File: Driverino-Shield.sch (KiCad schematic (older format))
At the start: 55 parts, among them P1 Power, P10 MOT, P11 HALL, P2 Analog, P3 Digital, P4 Digital, P5 CONN_01X01, P6 CONN_01X01, P7 CONN_01X01, P8 CONN_01X01, P9 PWR, U1 MCT8316Z

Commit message: Update
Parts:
- added JP2: VCC_SEL, Connector_PinHeader_1.27mm:PinHeader_1x02_P1.27mm_Vertical, symbol Device:Jumper
- C1, C10, C11, C12, C3, C4, C5, C6, C7, C8, C9: symbol device:C -> Driverino-Shield-rescue:C-device
- C2: symbol device:CP1 -> Driverino-Shield-rescue:CP1-device
- D1, D2, D3, D4: symbol device:LED -> Driverino-Shield-rescue:LED-device
- D5: symbol device:ZENER -> Driverino-Shield-rescue:ZENER-device
- F1: symbol device:FUSE -> Driverino-Shield-rescue:FUSE-device
- JP1: footprint Driverino-Shield:3JUMPER_0603 -> Connector_PinHeader_1.27mm:PinHeader_1x03_P1.27mm_Vertical; symbol device:JUMPER3 -> Driverino-Shield-rescue:JUMPER3-device
- L1: renamed from L2; symbol device:INDUCTOR_SMALL -> Driverino-Shield-rescue:INDUCTOR_SMALL-device
- P10: symbol conn:CONN_3 -> Driverino-Shield-rescue:CONN_3-conn
- P11: symbol conn:CONN_8 -> Driverino-Shield-rescue:CONN_8-conn
- P9: symbol conn:CONN_2 -> Driverino-Shield-rescue:CONN_2-conn
- R1, R10, R11, R12, R13, R14, R15, R16, R17, R18, R19, R2, R20, R21, R22, R23, R3, R4, R5, R6, R7, R8, R9: symbol device:R -> Driverino-Shield-rescue:R-device
- U1: symbol texas2:MCT8316Z -> Driverino-Shield-rescue:MCT8316Z-texas2
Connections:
- wire segments 237 -> 239

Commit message: Routing completed
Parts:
- C10, C11, C12, C4, C6: footprint Driverino-Shield:C_0603_1608Metric -> Capacitor_SMD:C_0402_1005Metric
- C3: footprint Driverino-Shield:C_0603_1608Metric -> Capacitor_SMD:C_1206_3216Metric
- JP2: symbol Device:Jumper -> Driverino-Shield-rescue:Jumper-Device
- R18, R19, R20, R21, R22, R23: footprint Resistor_SMD:R_0603_1608Metric -> Resistor_SMD:R_0402_1005Metric
- U1: symbol Driverino-Shield-rescue:MCT8316Z-texas2 -> Driverino-Shield-rescue:MCT8316Z-texas2-Driverino-Shield-rescue
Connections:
- net V: now also U1.16 (OUTB); no longer U1.16, (OUTB)

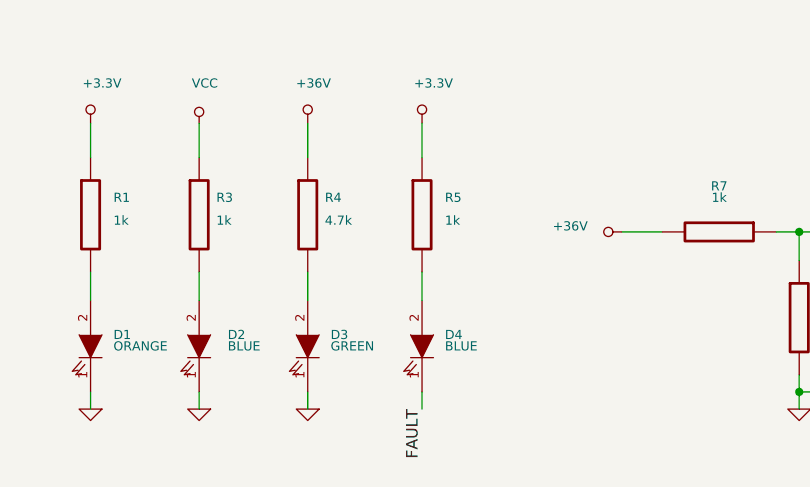
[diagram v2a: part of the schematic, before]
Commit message: Update
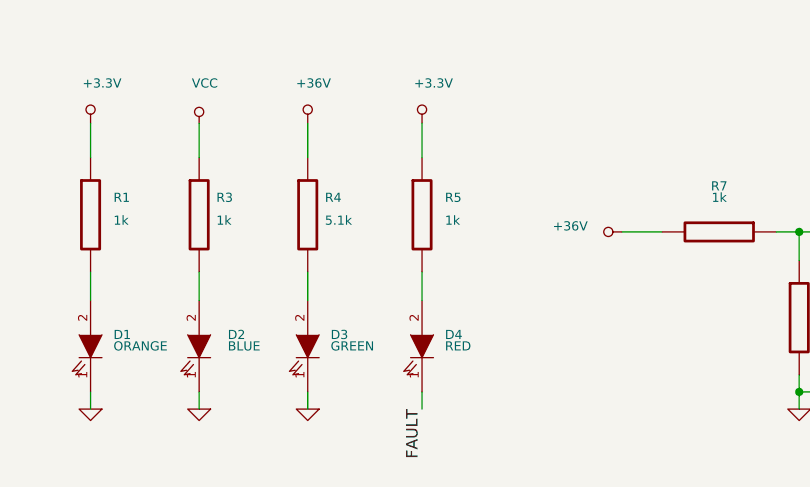
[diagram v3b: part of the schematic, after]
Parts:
- C1: Manufacturer (none) -> KEMET; Provider (none) -> RS; ProviderCode (none) -> 802-9967; manf# (none) -> C1206C226M8RACTU; mpn (none) -> C1206C226M8RACTU
- C10, C11, C12, C4: Manufacturer (none) -> TDK; Provider (none) -> RS; ProviderCode (none) -> 915-5635; manf# (none) -> CGA2B3X7R1V104K050BB; mpn (none) -> CGA2B3X7R1V104K050BB
- C2: Manufacturer (none) -> Panasonic; Provider (none) -> Mouser; ProviderCode (none) -> 667-EEE-FTV151XAV; manf# (none) -> EEE-FTV151XAV; mpn (none) -> EEE-FTV151XAV
- C3: Manufacturer (none) -> TDK; Provider (none) -> RS; ProviderCode (none) -> 915-5354; manf# (none) -> CGA5L1X7R1V106K160AE; mpn (none) -> CGA5L1X7R1V106K160AE
- C5, C7: Manufacturer (none) -> Yageo; Provider (none) -> RS; ProviderCode (none) -> 200-6596; manf# (none) -> CC0603KRX7R9BB105; mpn (none) -> CC0603KRX7R9BB105
- C6: Manufacturer (none) -> Murata; Provider (none) -> RS; ProviderCode (none) -> 723-4954; manf# (none) -> GCM155R71H103KA55D; mpn (none) -> GCM155R71H103KA55D
- C8, C9: Manufacturer (none) -> TDK; Provider (none) -> RS; ProviderCode (none) -> 788-2985; manf# (none) -> CGA3E2X7R1H104K080AA; mpn (none) -> CGA3E2X7R1H104K080AA
- D4: value BLUE -> RED
- D5: Manufacturer (none) -> Taiwan Semiconductor; Provider (none) -> Mouser; ProviderCode (none) -> 821-TSZU52C5V1RGG; manf# (none) -> TSZU52C5V1 RGG; mpn (none) -> TSZU52C5V1 RGG
- F1: Manufacturer (none) -> Bourns; Provider (none) -> Mouser; ProviderCode (none) -> 652-MF-ASML020/6-2; manf# (none) -> MF-ASML020/6-2; mpn (none) -> MF-ASML020/6-2
- JP1: Manufacturer (none) -> Samtec; Provider (none) -> Mouser; manf# (none) -> TMS-103-01-G-S; mpn (none) -> TMS-103-01-G-S
- JP2: Manufacturer (none) -> Samtec; Provider (none) -> Mouser; manf# (none) -> TMS-102-01-G-S; mpn (none) -> TMS-102-01-G-S
- L1: Manufacturer (none) -> Taiyo Yuden; Provider (none) -> Mouser; ProviderCode (none) -> 963-CBC3225T470KRV; manf# (none) -> CBC3225T470KRV; mpn (none) -> CBC3225T470KRV
- P1, P4: Manufacturer (none) -> Samtec; manf# (none) -> SSW-108-03-G-S; mpn (none) -> SSW-108-03-G-S
- P10: Manufacturer (none) -> Molex; manf# (none) -> 39773-0003; mpn (none) -> 39773-0003
- P11: Manufacturer (none) -> Molex; manf# (none) -> 53047-0810; mpn (none) -> 53047-0810
- P2: Manufacturer (none) -> Samtec; manf# (none) -> SSW-106-03-G-S; mpn (none) -> SSW-106-03-G-S
- P3: Manufacturer (none) -> Samtec; manf# (none) -> SSW-110-03-G-S; mpn (none) -> SSW-110-03-G-S
- P9: Manufacturer (none) -> Molex; manf# (none) -> 39773-0002; mpn (none) -> 39773-0002
- R1, R13, R3, R5, R7, R8: Manufacturer (none) -> Vishay; Provider (none) -> Mouser; ProviderCode (none) -> 71-CRCW06031K00FKEAC; manf# (none) -> CRCW06031K00FKEAC; mpn (none) -> CRCW06031K00FKEAC
- R10, R11, R12, R14, R15, R16, R17, R9: Manufacturer (none) -> Vishay; Provider (none) -> Mouser; ProviderCode (none) -> 71-CRCW06030000Z0EBC; manf# (none) -> CRCW06030000Z0EBC; mpn (none) -> CRCW06030000Z0EBC
- R18, R20, R22: Manufacturer (none) -> Vishay; Provider (none) -> Mouser; ProviderCode (none) -> 71-CRCW040210K0JNEDC; manf# (none) -> CRCW040210K0JNEDC; mpn (none) -> CRCW040210K0JNEDC
- R19, R21, R23: Manufacturer (none) -> Vishay; Provider (none) -> Mouser; ProviderCode (none) -> 71-RCC04020000Z0ED; manf# (none) -> RCC04020000Z0ED; mpn (none) -> RCC04020000Z0ED
- R2, R6: Manufacturer (none) -> Rohm; Provider (none) -> Mouser; ProviderCode (none) -> 755-ESR03EZPF5101; manf# (none) -> ESR03EZPF5101; mpn (none) -> ESR03EZPF5101
- R4: value 4.7k -> 5.1k; Manufacturer (none) -> Rohm; Provider (none) -> Mouser; ProviderCode (none) -> 755-ESR03EZPF5101; manf# (none) -> ESR03EZPF5101; mpn (none) -> ESR03EZPF5101
- U1: Manufacturer (none) -> TI; manf# (none) -> MCT8316Z; mpn (none) -> MCT8316Z

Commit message: .tsv file generated
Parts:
- D1: Manufacturer (none) -> 654-5795; Provider (none) -> RS; ProviderCode (none) -> OSRAM Opto; manf# (none) -> LO Q976; mpn (none) -> LO Q976
- D2: Manufacturer (none) -> 697-3610; Provider (none) -> RS; ProviderCode (none) -> OSRAM Opto; manf# (none) -> LB Q39G-N1OO-35-1; mpn (none) -> LB Q39G-N1OO-35-1
- D3: Manufacturer (none) -> 697-3715; Provider (none) -> RS; ProviderCode (none) -> OSRAM Opto; manf# (none) -> LT Q39G-Q1OO-25-1; mpn (none) -> LT Q39G-Q1OO-25-1
- D4: Manufacturer (none) -> 466-3728; Provider (none) -> RS; ProviderCode (none) -> Kingbright; manf# (none) -> KP-1608SRC-PRV; mpn (none) -> KP-1608SRC-PRV
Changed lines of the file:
@@
 F 2 "Driverino-Shield:LED_0603_1608Metric" H 5200 9200 60  0001 C CNN
 F 3 "" H 5200 9200 60  0000 C CNN
+F 4 "654-5795" H 5200 9200 50  0001 C CNN "Manufacturer"
+F 5 "RS" H 5200 9200 50  0001 C CNN "Provider"
+F 6 "OSRAM Opto" H 5200 9200 50  0001 C CNN "ProviderCode"
+F 7 "LO Q976" H 5200 9200 50  0001 C CNN "manf#"
+F 8 "LO Q976" H 5200 9200 50  0001 C CNN "mpn"
 	1    5200 9200
 	0    1    1    0
@@
 F 2 "Driverino-Shield:LED_0603_1608Metric" H 5675 9200 60  0001 C CNN
 F 3 "" H 5675 9200 60  0000 C CNN
+F 4 "697-3610" H 5675 9200 50  0001 C CNN "Manufacturer"
+F 5 "RS" H 5675 9200 50  0001 C CNN "Provider"
+F 6 "OSRAM Opto" H 5675 9200 50  0001 C CNN "ProviderCode"
+F 7 "LB Q39G-N1OO-35-1" H 5675 9200 50  0001 C CNN "manf#"
+F 8 "LB Q39G-N1OO-35-1" H 5675 9200 50  0001 C CNN "mpn"
 	1    5675 9200
 	0    1    1    0
@@
 F 2 "Driverino-Shield:LED_0603_1608Metric" H 6150 9200 60  0001 C CNN
 F 3 "" H 6150 9200 60  0000 C CNN
+F 4 "697-3715" H 6150 9200 50  0001 C CNN "Manufacturer"
+F 5 "RS" H 6150 9200 50  0001 C CNN "Provider"
+F 6 "OSRAM Opto" H 6150 9200 50  0001 C CNN "ProviderCode"
+F 7 "LT Q39G-Q1OO-25-1" H 6150 9200 50  0001 C CNN "manf#"
+F 8 "LT Q39G-Q1OO-25-1" H 6150 9200 50  0001 C CNN "mpn"
 	1    6150 9200
 	0    1    1    0
@@
 F 2 "Driverino-Shield:LED_0603_1608Metric" H 6650 9200 60  0001 C CNN
 F 3 "" H 6650 9200 60  0000 C CNN
+F 4 "466-3728" H 6650 9200 50  0001 C CNN "Manufacturer"
+F 5 "RS" H 6650 9200 50  0001 C CNN "Provider"
+F 6 "Kingbright" H 6650 9200 50  0001 C CNN "ProviderCode"
+F 7 "KP-1608SRC-PRV" H 6650 9200 50  0001 C CNN "manf#"
+F 8 "KP-1608SRC-PRV" H 6650 9200 50  0001 C CNN "mpn"
 	1    6650 9200
 	0    1    1    0

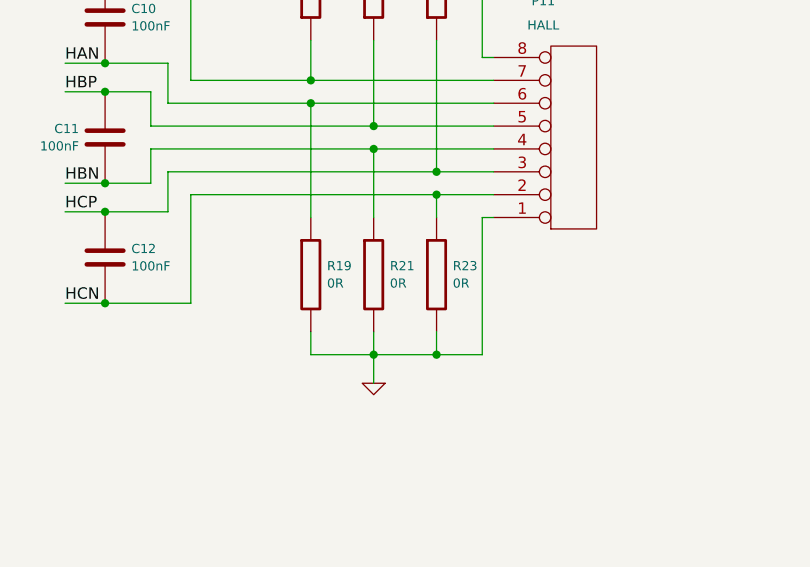
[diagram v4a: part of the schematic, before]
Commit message: Update BOM
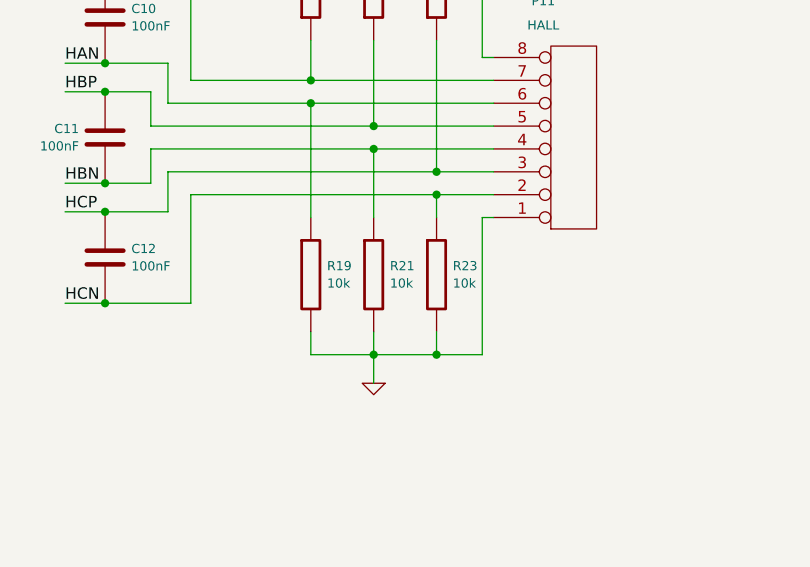
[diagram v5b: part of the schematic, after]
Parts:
- C10, C11, C12, P5, P6, P7, P8, R18, R20, R22: DNP (none) -> 1
- R19, R21, R23: value 0R -> 10k; DNP (none) -> 1; ProviderCode 71-RCC04020000Z0ED -> 71-CRCW040210K0JNEDC; manf# RCC04020000Z0ED -> CRCW040210K0JNEDC; mpn RCC04020000Z0ED -> CRCW040210K0JNEDC
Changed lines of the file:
@@
 F 2 "Socket_Arduino_Uno:Arduino_1pin" H 15571 724 20  0000 C CNN
 F 3 "" H 15650 650 50  0000 C CNN
+F 4 "1" H 15650 650 50  0001 C CNN "DNP"
 	1    15650 650
 	0    -1   -1   0
@@
 F 2 "Socket_Arduino_Uno:Arduino_1pin" H 15750 650 20  0001 C CNN
 F 3 "" H 15750 650 50  0000 C CNN
+F 4 "1" H 15750 650 50  0001 C CNN "DNP"
 	1    15750 650
 	0    -1   -1   0
@@
 F 2 "Socket_Arduino_Uno:Arduino_1pin" V 15850 650 20  0001 C CNN
 F 3 "" H 15850 650 50  0000 C CNN
+F 4 "1" H 15850 650 50  0001 C CNN "DNP"
 	1    15850 650
 	0    -1   -1   0
@@
 F 2 "Socket_Arduino_Uno:Arduino_1pin" H 15874 572 20  0000 C CNN
 F 3 "" H 15950 650 50  0000 C CNN
+F 4 "1" H 15950 650 50  0001 C CNN "DNP"
 	1    15950 650
 	0    -1   -1   0
@@
 F 7 "CGA2B3X7R1V104K050BB" H 13050 6425 50  0001 C CNN "manf#"
 F 8 "CGA2B3X7R1V104K050BB" H 13050 6425 50  0001 C CNN "mpn"
+F 9 "1" H 13050 6425 50  0001 C CNN "DNP"
 	1    13050 6425
 	-1   0    0    1
@@
 F 7 "CGA2B3X7R1V104K050BB" H 13050 6950 50  0001 C CNN "manf#"
 F 8 "CGA2B3X7R1V104K050BB" H 13050 6950 50  0001 C CNN "mpn"
+F 9 "1" H 13050 6950 50  0001 C CNN "DNP"
 	1    13050 6950
 	-1   0    0    1
@@
 F 7 "CGA2B3X7R1V104K050BB" H 13050 7475 50  0001 C CNN "manf#"
 F 8 "CGA2B3X7R1V104K050BB" H 13050 7475 50  0001 C CNN "mpn"
+F 9 "1" H 13050 7475 50  0001 C CNN "DNP"
 	1    13050 7475
 	-1   0    0    1
@@
 P 14225 7550
 F 0 "R21" H 14296 7588 40  0000 L CNN
-F 1 "0R" H 14296 7512 40  0000 L CNN
+F 1 "10k" H 14296 7512 40  0000 L CNN
 F 2 "Resistor_SMD:R_0402_1005Metric" V 14155 7550 30  0001 C CNN
 F 3 "" H 14225 7550 30  0000 C CNN
 F 4 "Vishay" H 14225 7550 50  0001 C CNN "Manufacturer"
 F 5 "Mouser" H 14225 7550 50  0001 C CNN "Provider"
-F 6 "71-RCC04020000Z0ED" H 14225 7550 50  0001 C CNN "ProviderCode"
-F 7 "RCC04020000Z0ED" H 14225 7550 50  0001 C CNN "manf#"
-F 8 "RCC04020000Z0ED" H 14225 7550 50  0001 C CNN "mpn"
+F 6 "71-CRCW040210K0JNEDC" H 14225 7550 50  0001 C CNN "ProviderCode"
+F 7 "CRCW040210K0JNEDC" H 14225 7550 50  0001 C CNN "manf#"
+F 8 "CRCW040210K0JNEDC" H 14225 7550 50  0001 C CNN "mpn"
+F 9 "1" H 14225 7550 50  0001 C CNN "DNP"
 	1    14225 7550
 	1    0    0    -1
@@
 P 13950 7550
 F 0 "R19" H 14021 7588 40  0000 L CNN
-F 1 "0R" H 14021 7512 40  0000 L CNN
+F 1 "10k" H 14021 7512 40  0000 L CNN
 F 2 "Resistor_SMD:R_0402_1005Metric" V 13880 7550 30  0001 C CNN
 F 3 "" H 13950 7550 30  0000 C CNN
 F 4 "Vishay" H 13950 7550 50  0001 C CNN "Manufacturer"
 F 5 "Mouser" H 13950 7550 50  0001 C CNN "Provider"
-F 6 "71-RCC04020000Z0ED" H 13950 7550 50  0001 C CNN "ProviderCode"
-F 7 "RCC04020000Z0ED" H 13950 7550 50  0001 C CNN "manf#"
-F 8 "RCC04020000Z0ED" H 13950 7550 50  0001 C CNN "mpn"
+F 6 "71-CRCW040210K0JNEDC" H 13950 7550 50  0001 C CNN "ProviderCode"
+F 7 "CRCW040210K0JNEDC" H 13950 7550 50  0001 C CNN "manf#"
+F 8 "CRCW040210K0JNEDC" H 13950 7550 50  0001 C CNN "mpn"
+F 9 "1" H 13950 7550 50  0001 C CNN "DNP"
 	1    13950 7550
 	1    0    0    -1
@@
 P 14500 7550
 F 0 "R23" H 14571 7588 40  0000 L CNN
-F 1 "0R" H 14571 7512 40  0000 L CNN
+F 1 "10k" H 14571 7512 40  0000 L CNN
 F 2 "Resistor_SMD:R_0402_1005Metric" V 14430 7550 30  0001 C CNN
 F 3 "" H 14500 7550 30  0000 C CNN
 F 4 "Vishay" H 14500 7550 50  0001 C CNN "Manufacturer"
 F 5 "Mouser" H 14500 7550 50  0001 C CNN "Provider"
-F 6 "71-RCC04020000Z0ED" H 14500 7550 50  0001 C CNN "ProviderCode"
-F 7 "RCC04020000Z0ED" H 14500 7550 50  0001 C CNN "manf#"
-F 8 "RCC04020000Z0ED" H 14500 7550 50  0001 C CNN "mpn"
+F 6 "71-CRCW040210K0JNEDC" H 14500 7550 50  0001 C CNN "ProviderCode"
+F 7 "CRCW040210K0JNEDC" H 14500 7550 50  0001 C CNN "manf#"
+F 8 "CRCW040210K0JNEDC" H 14500 7550 50  0001 C CNN "mpn"
+F 9 "1" H 14500 7550 50  0001 C CNN "DNP"
 	1    14500 7550
 	1    0    0    -1
@@
 F 7 "CRCW040210K0JNEDC" H 14500 6275 50  0001 C CNN "manf#"
 F 8 "CRCW040210K0JNEDC" H 14500 6275 50  0001 C CNN "mpn"
+F 9 "1" H 14500 6275 50  0001 C CNN "DNP"
 	1    14500 6275
 	1    0    0    1
@@
 F 7 "CRCW040210K0JNEDC" H 14225 6275 50  0001 C CNN "manf#"
 F 8 "CRCW040210K0JNEDC" H 14225 6275 50  0001 C CNN "mpn"
+F 9 "1" H 14225 6275 50  0001 C CNN "DNP"
 	1    14225 6275
 	1    0    0    1
@@
 F 7 "CRCW040210K0JNEDC" H 13950 6275 50  0001 C CNN "manf#"
 F 8 "CRCW040210K0JNEDC" H 13950 6275 50  0001 C CNN "mpn"
+F 9 "1" H 13950 6275 50  0001 C CNN "DNP"
 	1    13950 6275
 	1    0    0    1

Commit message: BOM Update
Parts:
- C1: Manf (none) -> KEMET; Manufacturer KEMET -> (none); OrderCode (none) -> 802-9967; ProviderCode 802-9967 -> (none)
- C10, C11, C12, C4: Manf (none) -> TDK; Manufacturer TDK -> (none); OrderCode (none) -> 915-5635; ProviderCode 915-5635 -> (none)
- C2: Manf (none) -> Panasonic; Manufacturer Panasonic -> (none); OrderCode (none) -> 667-EEE-FTV151XAV; ProviderCode 667-EEE-FTV151XAV -> (none)
- C3: Manf (none) -> TDK; Manufacturer TDK -> (none); OrderCode (none) -> 915-5354; ProviderCode 915-5354 -> (none)
- C5, C7: Manf (none) -> Yageo; Manufacturer Yageo -> (none); OrderCode (none) -> 200-6596; ProviderCode 200-6596 -> (none)
- C6: Manf (none) -> Murata; Manufacturer Murata -> (none); OrderCode (none) -> 723-4954; ProviderCode 723-4954 -> (none)
- C8, C9: Manf (none) -> TDK; Manufacturer TDK -> (none); OrderCode (none) -> 788-2985; ProviderCode 788-2985 -> (none)
- D1: Manf (none) -> OSRAM Opto; Manufacturer 654-5795 -> (none); OrderCode (none) -> 654-5795; ProviderCode OSRAM Opto -> (none)
- D2: Manf (none) -> OSRAM Opto; Manufacturer 697-3610 -> (none); OrderCode (none) -> 697-3610; ProviderCode OSRAM Opto -> (none)
- D3: Manf (none) -> OSRAM Opto; Manufacturer 697-3715 -> (none); OrderCode (none) -> 697-3715; ProviderCode OSRAM Opto -> (none)
- D4: Manf (none) -> Kingbright; Manufacturer 466-3728 -> (none); OrderCode (none) -> 466-3728; ProviderCode Kingbright -> (none)
- D5: Manf (none) -> Taiwan Semiconductor; Manufacturer Taiwan Semiconductor -> (none); OrderCode (none) -> 821-TSZU52C5V1RGG; ProviderCode 821-TSZU52C5V1RGG -> (none)
- F1: Manf (none) -> Bourns; Manufacturer Bourns -> (none); OrderCode (none) -> 652-MF-ASML020/6-2; ProviderCode 652-MF-ASML020/6-2 -> (none)
- JP1, JP2, P1, P2, P3, P4: Manf (none) -> Samtec; Manufacturer Samtec -> (none)
- L1: Manf (none) -> Taiyo Yuden; Manufacturer Taiyo Yuden -> (none); OrderCode (none) -> 963-CBC3225T470KRV; ProviderCode 963-CBC3225T470KRV -> (none)
- P10, P11, P9: Manf (none) -> Molex; Manufacturer Molex -> (none)
- R1, R13, R3, R5, R7, R8: Manf (none) -> Vishay; Manufacturer Vishay -> (none); OrderCode (none) -> 71-CRCW06031K00FKEAC; ProviderCode 71-CRCW06031K00FKEAC -> (none)
- R10, R11, R12, R14, R15, R16, R17, R9: Manf (none) -> Vishay; Manufacturer Vishay -> (none); OrderCode (none) -> 71-CRCW06030000Z0EBC; ProviderCode 71-CRCW06030000Z0EBC -> (none)
- R18, R19, R20, R21, R22, R23: Manf (none) -> Vishay; Manufacturer Vishay -> (none); OrderCode (none) -> 71-CRCW040210K0JNEDC; ProviderCode 71-CRCW040210K0JNEDC -> (none)
- R2, R4, R6: Manf (none) -> Rohm; Manufacturer Rohm -> (none); OrderCode (none) -> 755-ESR03EZPF5101; ProviderCode 755-ESR03EZPF5101 -> (none)
- U1: Manf (none) -> TI; Manufacturer TI -> (none)

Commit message: Updated BOM
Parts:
- C10, C11, C12, P5, P6, P7, P8, R18, R19, R20, R21, R22, R23: DNF (none) -> 1; DNP 1 -> (none)
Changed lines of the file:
@@
 F 2 "Socket_Arduino_Uno:Arduino_1pin" H 15571 724 20  0000 C CNN
 F 3 "" H 15650 650 50  0000 C CNN
-F 4 "1" H 15650 650 50  0001 C CNN "DNP"
+F 4 "1" H 15650 650 50  0001 C CNN "DNF"
 	1    15650 650
 	0    -1   -1   0
@@
 F 2 "Socket_Arduino_Uno:Arduino_1pin" H 15750 650 20  0001 C CNN
 F 3 "" H 15750 650 50  0000 C CNN
-F 4 "1" H 15750 650 50  0001 C CNN "DNP"
+F 4 "1" H 15750 650 50  0001 C CNN "DNF"
 	1    15750 650
 	0    -1   -1   0
@@
 F 2 "Socket_Arduino_Uno:Arduino_1pin" V 15850 650 20  0001 C CNN
 F 3 "" H 15850 650 50  0000 C CNN
-F 4 "1" H 15850 650 50  0001 C CNN "DNP"
+F 4 "1" H 15850 650 50  0001 C CNN "DNF"
 	1    15850 650
 	0    -1   -1   0
@@
 F 2 "Socket_Arduino_Uno:Arduino_1pin" H 15874 572 20  0000 C CNN
 F 3 "" H 15950 650 50  0000 C CNN
-F 4 "1" H 15950 650 50  0001 C CNN "DNP"
+F 4 "1" H 15950 650 50  0001 C CNN "DNF"
 	1    15950 650
 	0    -1   -1   0
@@
 F 7 "CGA2B3X7R1V104K050BB" H 13050 6425 50  0001 C CNN "manf#"
 F 8 "CGA2B3X7R1V104K050BB" H 13050 6425 50  0001 C CNN "mpn"
-F 9 "1" H 13050 6425 50  0001 C CNN "DNP"
+F 9 "1" H 13050 6425 50  0001 C CNN "DNF"
 	1    13050 6425
 	-1   0    0    1
@@
 F 7 "CGA2B3X7R1V104K050BB" H 13050 6950 50  0001 C CNN "manf#"
 F 8 "CGA2B3X7R1V104K050BB" H 13050 6950 50  0001 C CNN "mpn"
-F 9 "1" H 13050 6950 50  0001 C CNN "DNP"
+F 9 "1" H 13050 6950 50  0001 C CNN "DNF"
 	1    13050 6950
 	-1   0    0    1
@@
 F 7 "CGA2B3X7R1V104K050BB" H 13050 7475 50  0001 C CNN "manf#"
 F 8 "CGA2B3X7R1V104K050BB" H 13050 7475 50  0001 C CNN "mpn"
-F 9 "1" H 13050 7475 50  0001 C CNN "DNP"
+F 9 "1" H 13050 7475 50  0001 C CNN "DNF"
 	1    13050 7475
 	-1   0    0    1
@@
 F 7 "CRCW040210K0JNEDC" H 14225 7550 50  0001 C CNN "manf#"
 F 8 "CRCW040210K0JNEDC" H 14225 7550 50  0001 C CNN "mpn"
-F 9 "1" H 14225 7550 50  0001 C CNN "DNP"
+F 9 "1" H 14225 7550 50  0001 C CNN "DNF"
 	1    14225 7550
 	1    0    0    -1
@@
 F 7 "CRCW040210K0JNEDC" H 13950 7550 50  0001 C CNN "manf#"
 F 8 "CRCW040210K0JNEDC" H 13950 7550 50  0001 C CNN "mpn"
-F 9 "1" H 13950 7550 50  0001 C CNN "DNP"
+F 9 "1" H 13950 7550 50  0001 C CNN "DNF"
 	1    13950 7550
 	1    0    0    -1
@@
 F 7 "CRCW040210K0JNEDC" H 14500 7550 50  0001 C CNN "manf#"
 F 8 "CRCW040210K0JNEDC" H 14500 7550 50  0001 C CNN "mpn"
-F 9 "1" H 14500 7550 50  0001 C CNN "DNP"
+F 9 "1" H 14500 7550 50  0001 C CNN "DNF"
 	1    14500 7550
 	1    0    0    -1
@@
 F 7 "CRCW040210K0JNEDC" H 14500 6275 50  0001 C CNN "manf#"
 F 8 "CRCW040210K0JNEDC" H 14500 6275 50  0001 C CNN "mpn"
-F 9 "1" H 14500 6275 50  0001 C CNN "DNP"
+F 9 "1" H 14500 6275 50  0001 C CNN "DNF"
 	1    14500 6275
 	1    0    0    1
@@
 F 7 "CRCW040210K0JNEDC" H 14225 6275 50  0001 C CNN "manf#"
 F 8 "CRCW040210K0JNEDC" H 14225 6275 50  0001 C CNN "mpn"
-F 9 "1" H 14225 6275 50  0001 C CNN "DNP"
+F 9 "1" H 14225 6275 50  0001 C CNN "DNF"
 	1    14225 6275
 	1    0    0    1
@@
 F 7 "CRCW040210K0JNEDC" H 13950 6275 50  0001 C CNN "manf#"
 F 8 "CRCW040210K0JNEDC" H 13950 6275 50  0001 C CNN "mpn"
-F 9 "1" H 13950 6275 50  0001 C CNN "DNP"
+F 9 "1" H 13950 6275 50  0001 C CNN "DNF"
 	1    13950 6275
 	1    0    0    1
